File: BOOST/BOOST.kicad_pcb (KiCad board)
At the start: 4 copper layers, 27.9 x 17.8 mm, 25 parts, among them J1 JST, U1 MCP73831-2-OT, U2 TPS61090

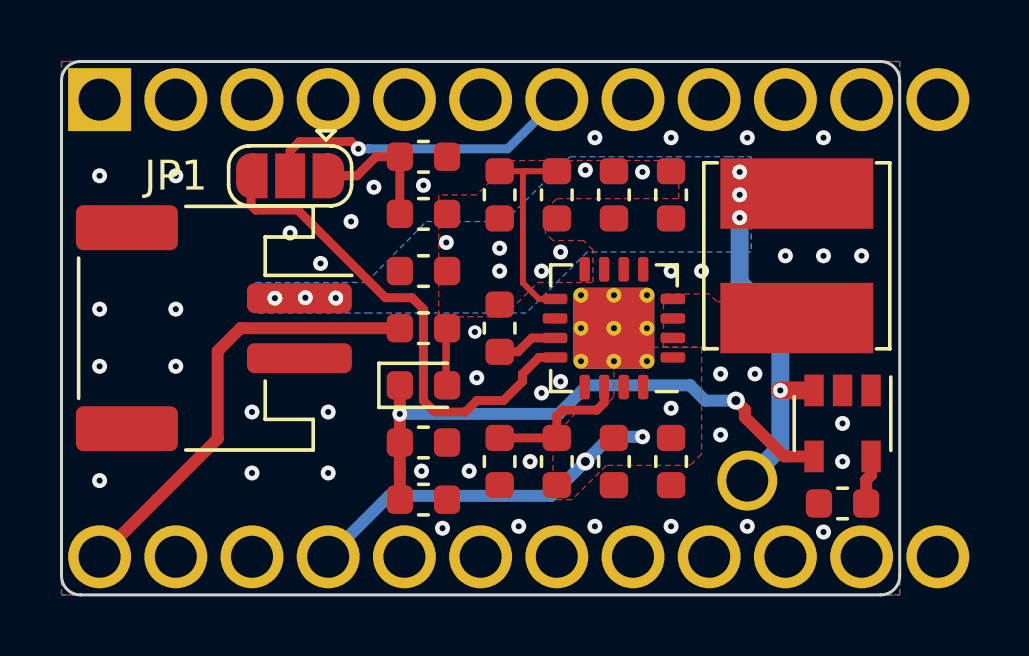
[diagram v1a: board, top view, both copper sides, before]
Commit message: major cleanup and fixes
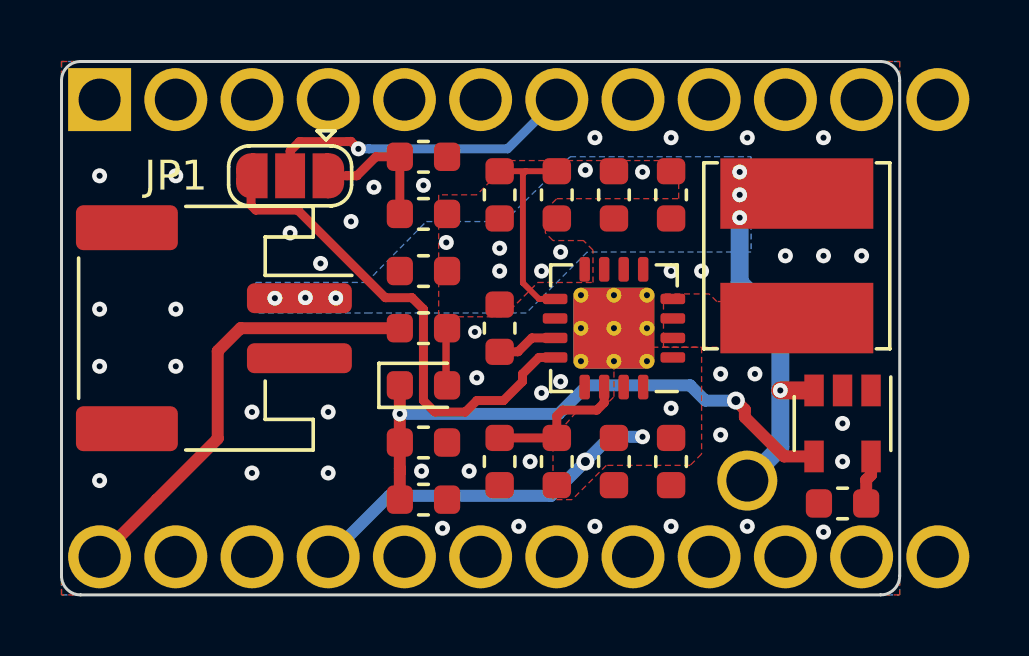
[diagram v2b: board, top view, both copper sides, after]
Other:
- net class Default removed
- net class Power removed
- net class small removed
- net class tiny removed
